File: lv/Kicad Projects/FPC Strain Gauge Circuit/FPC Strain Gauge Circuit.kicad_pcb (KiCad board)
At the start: 4 copper layers, 15 x 10 mm, 24 parts, among them U1 INA333xxDGK, U2 OPA333xxDBV, U3 ADS1220IRVAR

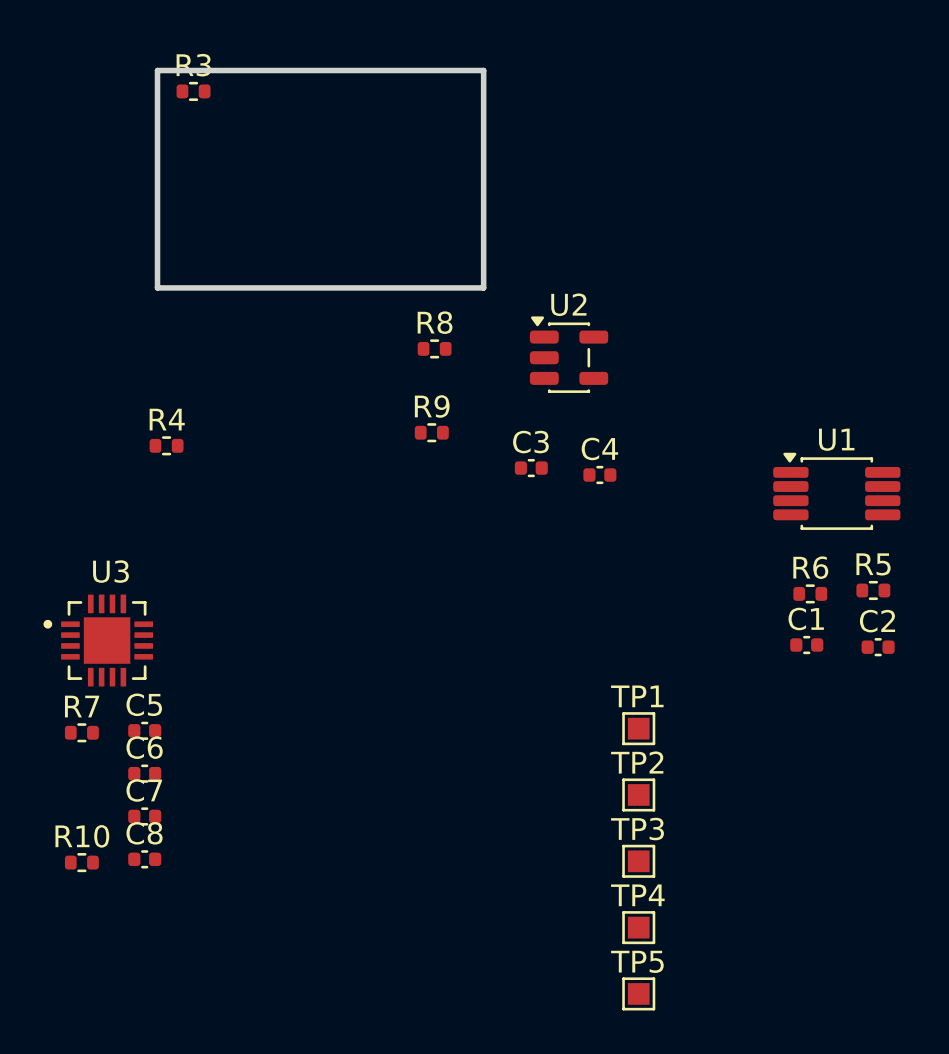
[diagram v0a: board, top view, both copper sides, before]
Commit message: Finish Circuit PCB
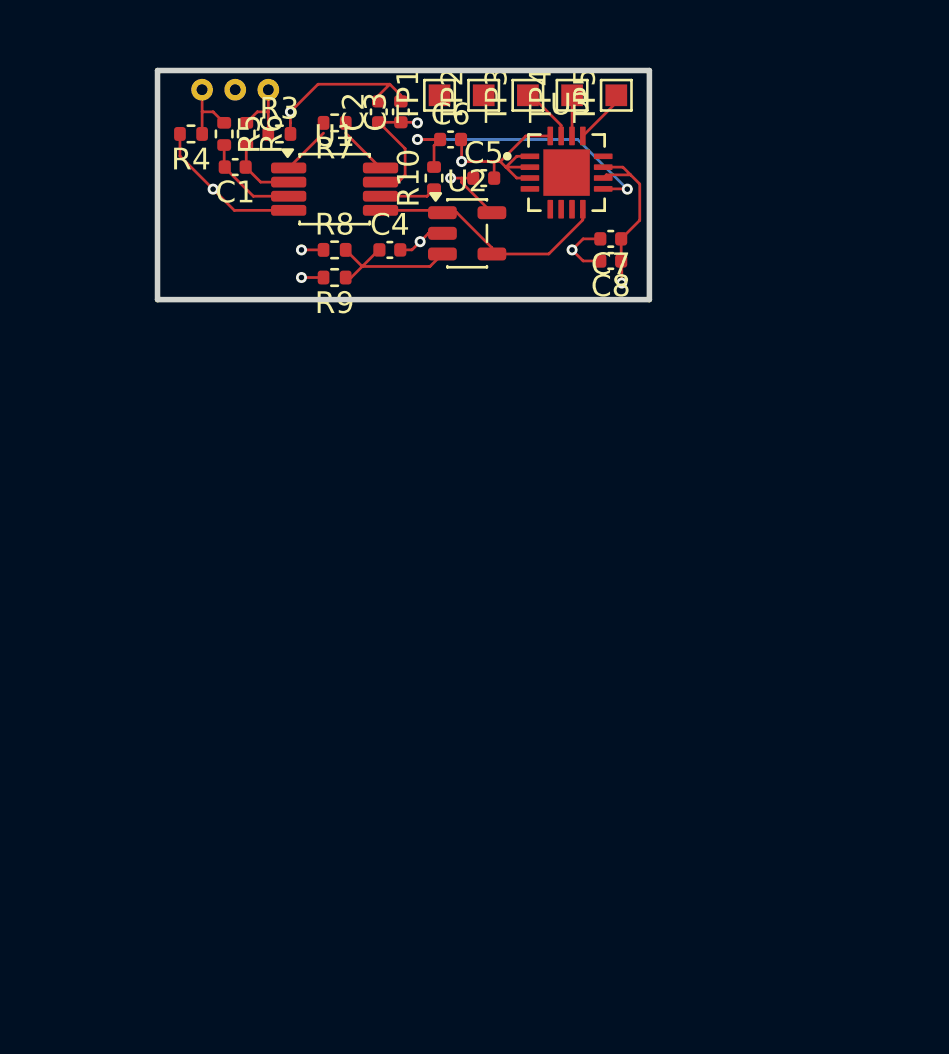
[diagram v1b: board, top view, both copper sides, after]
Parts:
- added ?: , , F.Cu at (122.4, 67.6)
- added ?: , , F.Cu at (124.0, 67.6)
- added ?: , , F.Cu at (125.5, 67.6)
- moved TP5 41.3 mm to (141.5, 67.8), turned to 90 degrees
- moved TP4 38.4 mm to (139.4, 67.8), turned to 90 degrees
- moved R5 36.5 mm to (123.4, 69.6), turned to -90 degrees
- moved TP3 35.6 mm to (137.4, 67.8), turned to 90 degrees
- moved R10 35.4 mm to (133.1, 71.6), turned to 90 degrees
- moved C8 34.9 mm to (141.2, 75.4), turned to 180 degrees
- moved C1 34.3 mm to (124.0, 71.1), turned to 180 degrees
- moved C7 34.1 mm to (141.2, 74.4), turned to 180 degrees
- moved C2 33.7 mm to (130.6, 68.6), turned to 90 degrees
- moved R6 33.5 mm to (124.5, 69.6), turned to -90 degrees
- moved TP2 33.0 mm to (135.4, 67.8), turned to 90 degrees
- moved C6 32.4 mm to (133.9, 69.8)
- moved TP1 30.5 mm to (133.3, 67.8), turned to 90 degrees
- moved R7 30.4 mm to (128.5, 69.1), turned to 180 degrees
- moved U3 30.2 mm to (139.2, 71.4)
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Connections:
- net /BRIDGE_N renamed R1
- net /BRIDGE_P renamed R2
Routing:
- net AGND: track 0.00 -> 31.9 mm, vias 0 -> 6
- net +3V3_A: track 0.00 -> 18.5 mm, vias 0 -> 4
- net /LOAD_SIGNAL: track 0.00 -> 14.1 mm, vias 0 -> 2
- net /VREF_1V65: track 0.00 -> 11.5 mm
- net /VREF_RAW: track 0.00 -> 7.08 mm
- net Net-(U1-+): track 0.00 -> 4.54 mm
- net Net-(U1--): track 0.00 -> 3.29 mm
- net R1: track 0.00 -> 3.25 mm
- net R2: track 0.00 -> 3.25 mm
- net Net-(R10-Pad1): track 0.00 -> 2.59 mm
- net /ADC_SCLK: track 0.00 -> 2.59 mm
- net /ADC_MISO: track 0.00 -> 2.51 mm
- net Net-(R7-Pad1): track 0.00 -> 2.27 mm
- net Net-(R7-Pad2): track 0.00 -> 2.27 mm
- net /ADC_MOSI: track 0.00 -> 1.87 mm
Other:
- board size 15 x 10 mm -> 22.6 x 10.5 mm
